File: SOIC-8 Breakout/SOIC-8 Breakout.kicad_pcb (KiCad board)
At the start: 2 copper layers, 23.1 x 15.5 mm, 0 parts

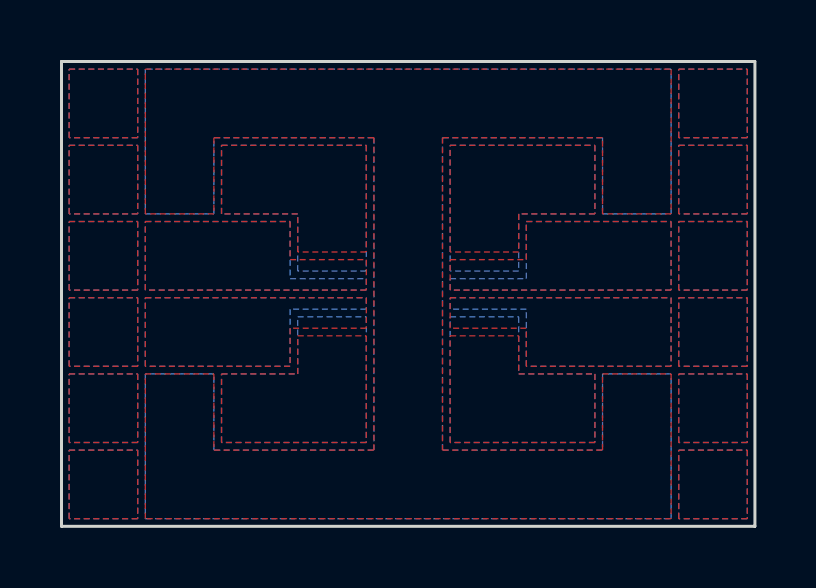
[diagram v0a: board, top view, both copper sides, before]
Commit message: Updated Files
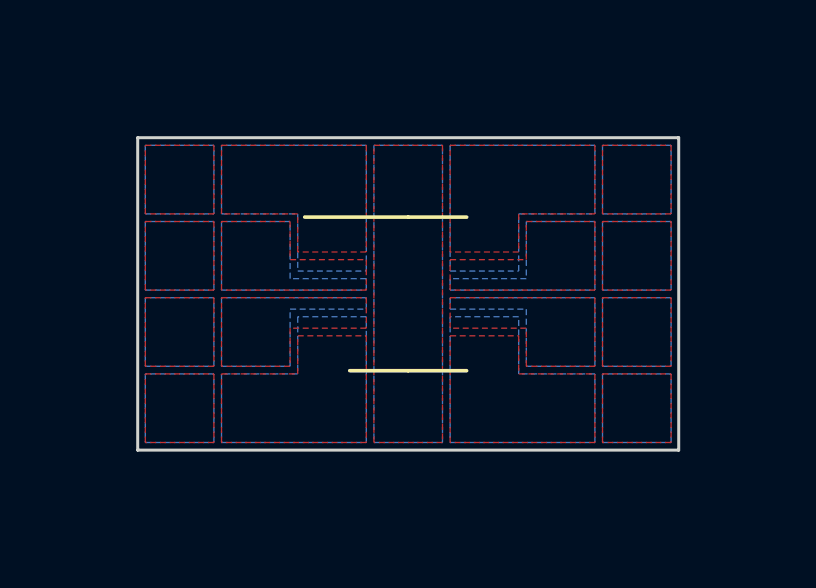
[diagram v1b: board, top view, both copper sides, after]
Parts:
- added REF**: SOIC-8_3.9x4.9mm_P1.27mm, Package_SO:SOIC-8_3.9x4.9mm_P1.27mm, F.Cu at (152.4, 101.6)
- added REF**: C_0603_1608Metric, Capacitor_SMD:C_0603_1608Metric, B.Cu at (153.7, 105.4)
- added REF**: C_0603_1608Metric, Capacitor_SMD:C_0603_1608Metric, B.Cu at (158.8, 100.3)
- added REF**: C_0603_1608Metric, Capacitor_SMD:C_0603_1608Metric, B.Cu at (151.1, 97.8)
- added REF**: R_0603_1608Metric, Resistor_SMD:R_0603_1608Metric, B.Cu at (158.8, 105.4)
- added REF**: R_0603_1608Metric, Resistor_SMD:R_0603_1608Metric, B.Cu at (146.1, 97.8)
- added REF**: C_0603_1608Metric, Capacitor_SMD:C_0603_1608Metric, B.Cu at (158.8, 102.9)
- added REF**: C_0603_1608Metric, Capacitor_SMD:C_0603_1608Metric, B.Cu at (151.1, 105.4)
- added REF**: R_0603_1608Metric, Resistor_SMD:R_0603_1608Metric, B.Cu at (146.1, 105.4)
- added REF**: C_0603_1608Metric, Capacitor_SMD:C_0603_1608Metric, B.Cu at (146.1, 102.9)
- added REF**: R_0603_1608Metric, Resistor_SMD:R_0603_1608Metric, B.Cu at (158.8, 97.8)
- added REF**: MSOP-8_3x3mm_P0.65mm, Package_SO:MSOP-8_3x3mm_P0.65mm, B.Cu at (152.4, 101.6)
- added REF**: C_0603_1608Metric, Capacitor_SMD:C_0603_1608Metric, B.Cu at (146.1, 100.3)
- added REF**: C_0603_1608Metric, Capacitor_SMD:C_0603_1608Metric, B.Cu at (153.7, 97.8)
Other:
- board size 23.1 x 15.5 mm -> 18 x 10.4 mm
